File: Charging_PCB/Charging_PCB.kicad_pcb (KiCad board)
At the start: 2 copper layers, 80 x 59.5 mm, 17 parts, among them K3 Relay_SPDT_Omron_G2RL-1, K4 Relay_SPDT_Omron_G2RL-1, Q3 Q_PMOS_GSD, Q4 Q_PMOS_GSD, U112 641964-1, U113 641964-1, U114 641964-1

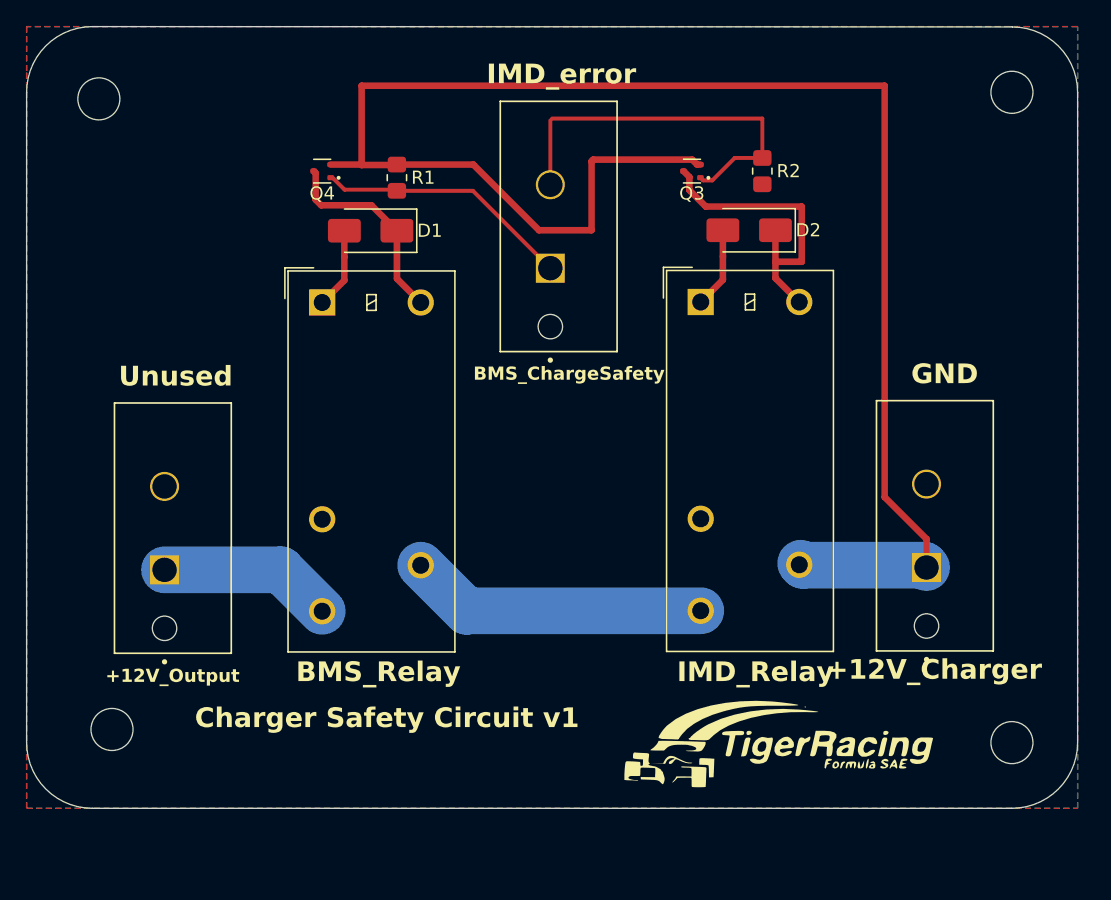
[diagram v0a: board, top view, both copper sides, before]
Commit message: CHARGE READY
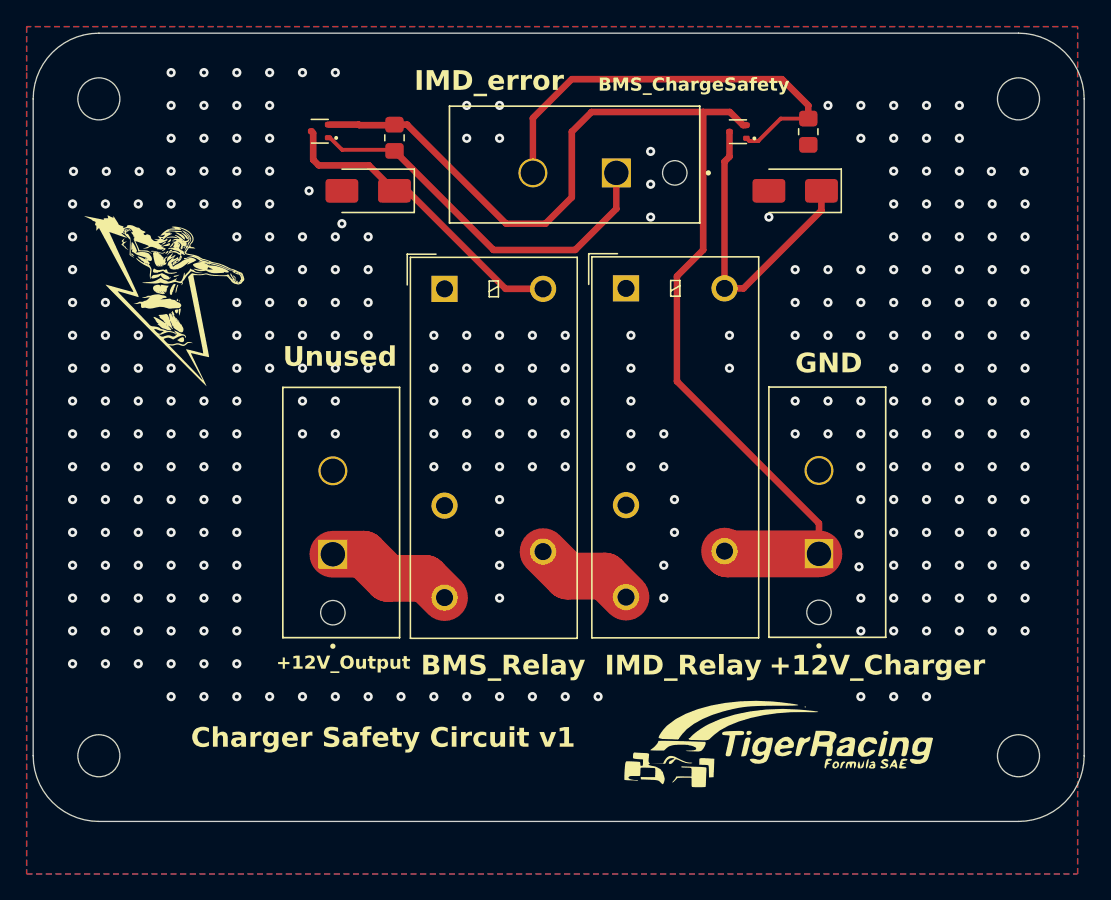
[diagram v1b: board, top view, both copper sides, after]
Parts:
- added G***: LOGO, LOGO, F.Cu at (117.0, 94.5)
- moved U103 12.9 mm to (129.8, 114.2)
- moved K101 9.37 mm to (138.3, 94.0)
- moved U101 8.82 mm to (151.4, 85.1), turned to 180 degrees
- moved U102 8.25 mm to (166.8, 114.1)
- moved K102 5.78 mm to (152.1, 93.9)
- moved D102 4.61 mm to (165.0, 86.5)
- moved Q102 4.61 mm to (160.6, 82.0)
- moved R102 4.61 mm to (166.0, 82.0)
- moved D101 3.04 mm to (132.5, 86.5)
- moved Q101 3.04 mm to (128.8, 82.0)
- moved R101 3.04 mm to (134.5, 82.5)
- moved H104 2.24 mm to (112.0, 129.5)
- moved H102 1.12 mm to (182.0, 129.5)
- moved H101 0.71 mm to (182.0, 79.5)
- renumbered D1 to D101, D2 to D102, H103 to H102, H102 to H103, K3 to K101, K4 to K102, Q4 to Q101, Q3 to Q102, R1 to R101, R2 to R102, U113 to U101, U112 to U102, U114 to U103
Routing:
- net +12V: track 129.4 -> 88.2 mm
- net Net-(K101-Pad11): track 22.8 -> 7.75 mm
- net GND: track 12.3 -> 0.00 mm, vias 0 -> 295
- net /BMS_CSO: track 19.6 -> 29.5 mm
- net Net-(D101-K): track 15.6 -> 23.8 mm
- net /IMD_Error: track 29.6 -> 33.7 mm
- net /+12_Relay: track 13.3 -> 9.87 mm
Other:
- board size 80 x 59.5 mm -> 80 x 60 mm
